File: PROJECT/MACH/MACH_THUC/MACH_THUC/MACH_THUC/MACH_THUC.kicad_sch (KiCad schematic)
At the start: 66 parts, among them K1 SANYOU_SRD_Form_C, K2 SANYOU_SRD_Form_C, Q1 2SB688, Q2 BC547, Q3 BC547, U1 LM7805_TO220, U2 DS1307+, U3 LCD-016N002L, U4 PCF8574, U5 PC817, U6 PC817, Y1 Crystal 20M, Y2 Crystal 32.768KHz

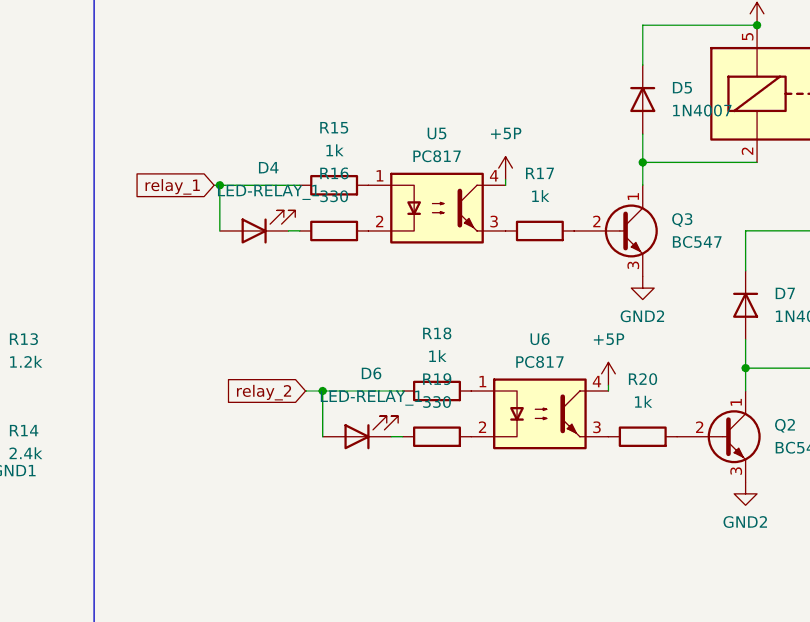
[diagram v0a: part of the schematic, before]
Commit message: update code
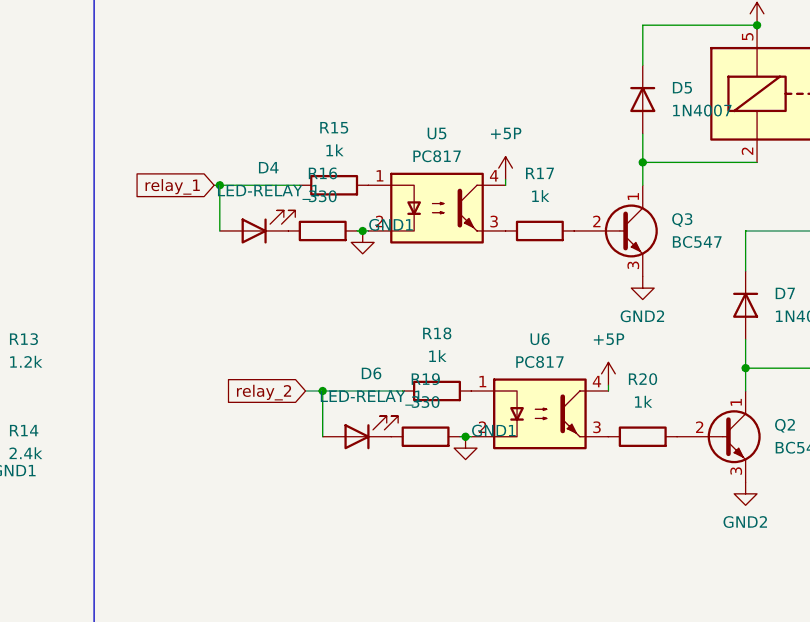
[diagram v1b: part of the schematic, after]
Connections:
- net GND1: now also R16.2, R19.2, U5.2, U6.2
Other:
- moved on the sheet: R16, R19
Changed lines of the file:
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@@
   (junction (at 59.69 121.285) (diameter 0) (color 0 0 0 0)
   )
+  (junction (at 194.31 151.765) (diameter 0) (color 0 0 0 0)
+  )
   (junction (at 227.33 29.21) (diameter 0) (color 0 0 0 0)
   )
@@
   (junction (at 212.725 61.595) (diameter 0) (color 0 0 0 0)
   )
+  (junction (at 182.88 128.905) (diameter 0) (color 0 0 0 0)
+  )
   (junction (at 38.1 31.115) (diameter 0) (color 0 0 0 0)
   )
@@
     (stroke (width 0) (type default))
   )
+  (wire (pts (xy 193.675 151.765) (xy 194.31 151.765))
+    (stroke (width 0) (type default))
+  )
   (wire (pts (xy 188.595 80.01) (xy 188.595 87.63))
     (stroke (width 0) (type default))
@@
     (stroke (width 0) (type default))
   )
+  (wire (pts (xy 194.31 151.765) (xy 194.945 151.765))
+    (stroke (width 0) (type default))
+  )
   (wire (pts (xy 148.59 43.815) (xy 152.4 43.815))
     (stroke (width 0) (type default))
@@
     (stroke (width 0) (type default))
   )
+  (wire (pts (xy 182.88 128.905) (xy 183.515 128.905))
+    (stroke (width 0) (type default))
+  )
   (wire (pts (xy 48.26 51.435) (xy 48.26 60.96))
     (stroke (width 0) (type default))
@@
     (stroke (width 0) (type default))
   )
+  (wire (pts (xy 182.245 128.905) (xy 182.88 128.905))
+    (stroke (width 0) (type default))
+  )
   (wire (pts (xy 46.99 163.83) (xy 49.53 163.83))
     (stroke (width 0) (type default))
@@
     (stroke (width 0) (type default))
   )
-  (wire (pts (xy 186.055 151.765) (xy 187.325 151.765))
-    (stroke (width 0) (type default))
-  )
   (wire (pts (xy 120.015 29.21) (xy 120.015 31.115))
     (stroke (width 0) (type default))
@@
     (stroke (width 0) (type default))
   )
-  (wire (pts (xy 174.625 128.905) (xy 175.895 128.905))
-    (stroke (width 0) (type default))
-  )
   (wire (pts (xy 104.14 38.735) (xy 104.14 41.275))
     (stroke (width 0) (type default))
@@
     )
   )
-  (symbol (lib_id "Device:R") (at 191.135 151.765 90) (unit 1)
+  (symbol (lib_id "Device:R") (at 189.865 151.765 90) (unit 1)
     (in_bom yes) (on_board yes) (dnp no) (fields_autoplaced)
-    (property "Reference" "R19" (at 191.135 145.415 90)
+    (property "Reference" "R19" (at 189.865 145.415 90)
       (effects (font (size 1.27 1.27)))
     )
-    (property "Value" "330" (at 191.135 147.955 90)
+    (property "Value" "330" (at 189.865 147.955 90)
       (effects (font (size 1.27 1.27)))
     )
-    (property "Footprint" "library_thuan_footprint:RES_DEFAULT" (at 191.135 153.543 90)
+    (property "Footprint" "library_thuan_footprint:RES_DEFAULT" (at 189.865 153.543 90)
       (effects (font (size 1.27 1.27)) hide)
     )
-    (property "Datasheet" "https://www.thegioiic.com/dien-tro-330-kohm-1-4w-5-4-vong-mau" (at 191.135 151.765 0)
+    (property "Datasheet" "https://www.thegioiic.com/dien-tro-330-kohm-1-4w-5-4-vong-mau" (at 189.865 151.765 0)
       (effects (font (size 1.27 1.27)) hide)
     )
@@
     )
   )
+  (symbol (lib_id "power:GND1") (at 194.31 151.765 0) (unit 1)
+    (in_bom yes) (on_board yes) (dnp no)
+    (property "Reference" "#PWR046" (at 194.31 158.115 0)
+      (effects (font (size 1.27 1.27)) hide)
+    )
+    (property "Value" "GND1" (at 197.485 151.13 0)
+      (effects (font (size 1.27 1.27)))
+    )
+    (property "Footprint" "" (at 194.31 151.765 0)
+      (effects (font (size 1.27 1.27)) hide)
+    )
+    (property "Datasheet" "" (at 194.31 151.765 0)
+      (effects (font (size 1.27 1.27)) hide)
+    )
+    (pin "1")
+    (instances
+      (project "MACH_THUC"
+        (path "/fa9b692b-a58b-4246-a447-a74a2194b64e"
+          (reference "#PWR046") (unit 1)
+        )
+      )
+    )
+  )
   (symbol (lib_id "power:+5V") (at 107.95 154.94 90) (unit 1)
     (in_bom yes) (on_board yes) (dnp no) (fields_autoplaced)
@@
     )
   )
-  (symbol (lib_id "Device:R") (at 179.705 128.905 90) (unit 1)
+  (symbol (lib_id "Device:R") (at 178.435 128.905 90) (unit 1)
     (in_bom yes) (on_board yes) (dnp no) (fields_autoplaced)
-    (property "Reference" "R16" (at 179.705 122.555 90)
+    (property "Reference" "R16" (at 178.435 122.555 90)
       (effects (font (size 1.27 1.27)))
     )
-    (property "Value" "330" (at 179.705 125.095 90)
+    (property "Value" "330" (at 178.435 125.095 90)
       (effects (font (size 1.27 1.27)))
     )
-    (property "Footprint" "library_thuan_footprint:RES_DEFAULT" (at 179.705 130.683 90)
+    (property "Footprint" "library_thuan_footprint:RES_DEFAULT" (at 178.435 130.683 90)
       (effects (font (size 1.27 1.27)) hide)
     )
-    (property "Datasheet" "https://www.thegioiic.com/dien-tro-330-kohm-1-4w-5-4-vong-mau" (at 179.705 128.905 0)
+    (property "Datasheet" "https://www.thegioiic.com/dien-tro-330-kohm-1-4w-5-4-vong-mau" (at 178.435 128.905 0)
       (effects (font (size 1.27 1.27)) hide)
     )
@@
         )
       )
+    )
+  )
+  (symbol (lib_id "power:GND1") (at 182.88 128.905 0) (unit 1)
+    (in_bom yes) (on_board yes) (dnp no)
+    (property "Reference" "#PWR045" (at 182.88 135.255 0)
+      (effects (font (size 1.27 1.27)) hide)
+    )
+    (property "Value" "GND1" (at 186.055 128.27 0)
+      (effects (font (size 1.27 1.27)))
+    )
+    (property "Footprint" "" (at 182.88 128.905 0)
+      (effects (font (size 1.27 1.27)) hide)
+    )
+    (property "Datasheet" "" (at 182.88 128.905 0)
+      (effects (font (size 1.27 1.27)) hide)
+    )
+    (pin "1")
+    (instances
+      (project "MACH_THUC"
+        (path "/fa9b692b-a58b-4246-a447-a74a2194b64e"
+          (reference "#PWR045") (unit 1)
+        )
+      )
